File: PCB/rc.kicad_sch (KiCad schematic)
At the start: 5 parts, among them J1 USB_C_Receptacle_USB2.0_16P, J2 USB_A, J3 Conn_01x07_Pin, U1 ESP32-S3-WROOM-1U, U2 MAX3421EEHJ+T

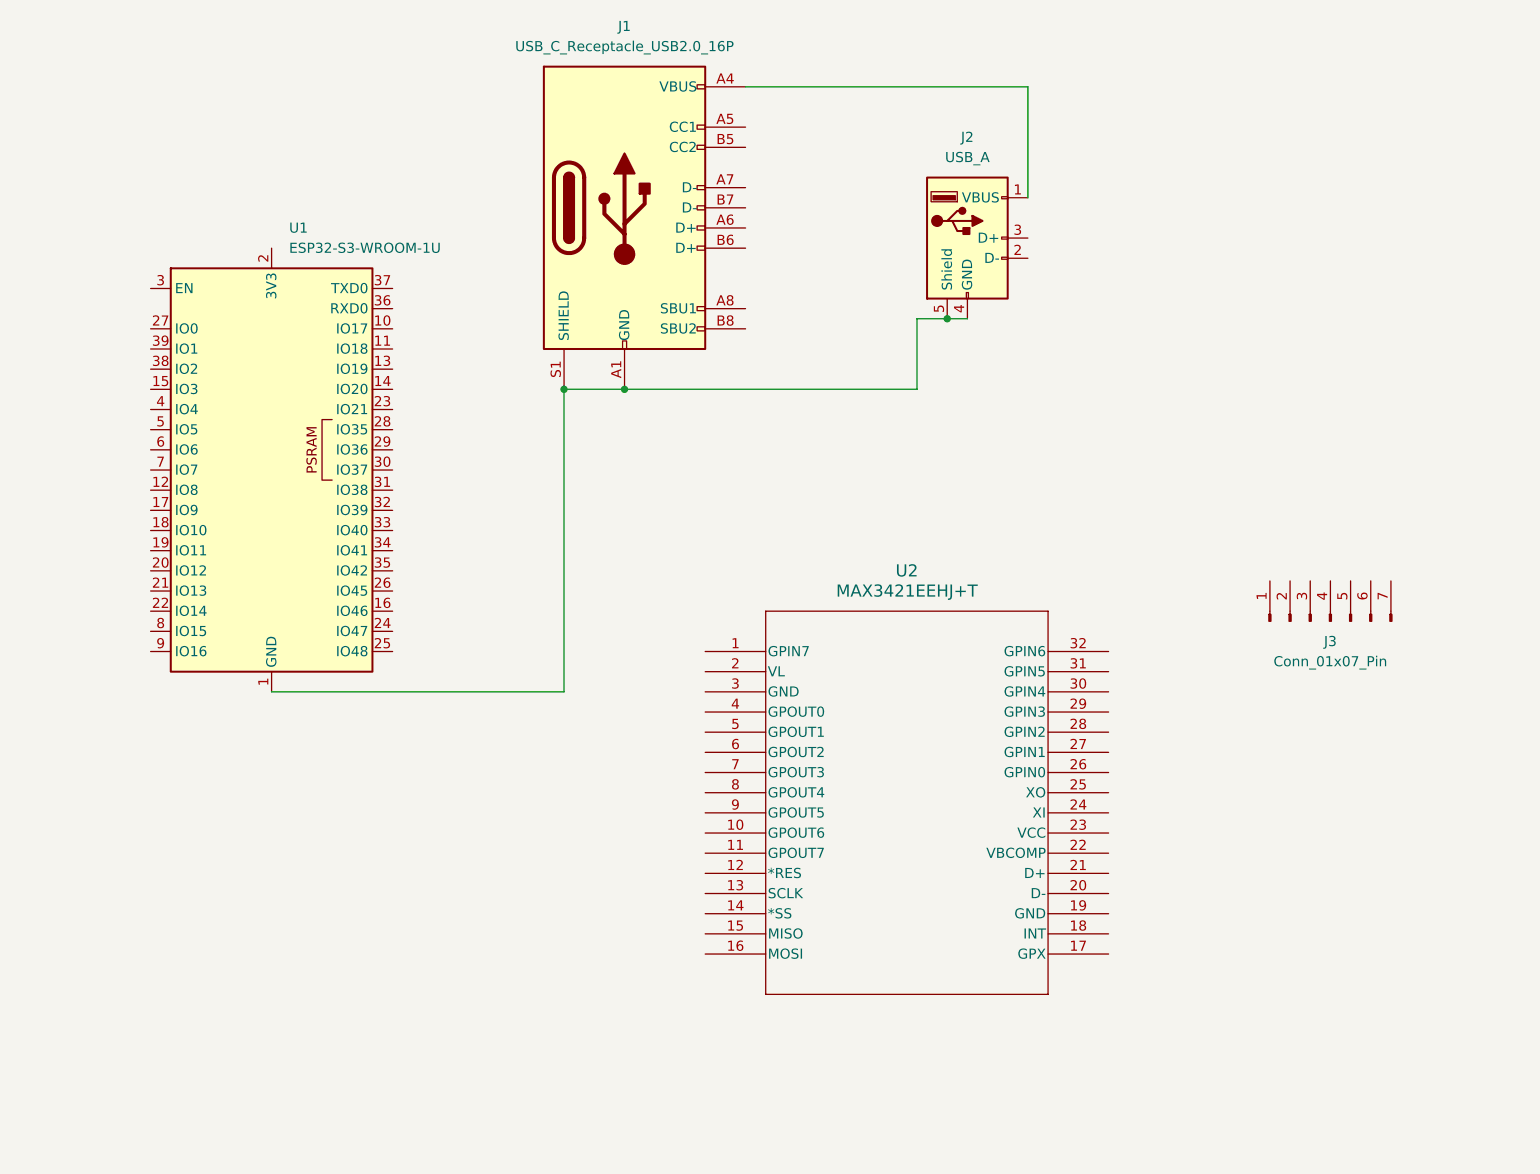
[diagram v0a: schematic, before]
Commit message: pcb init
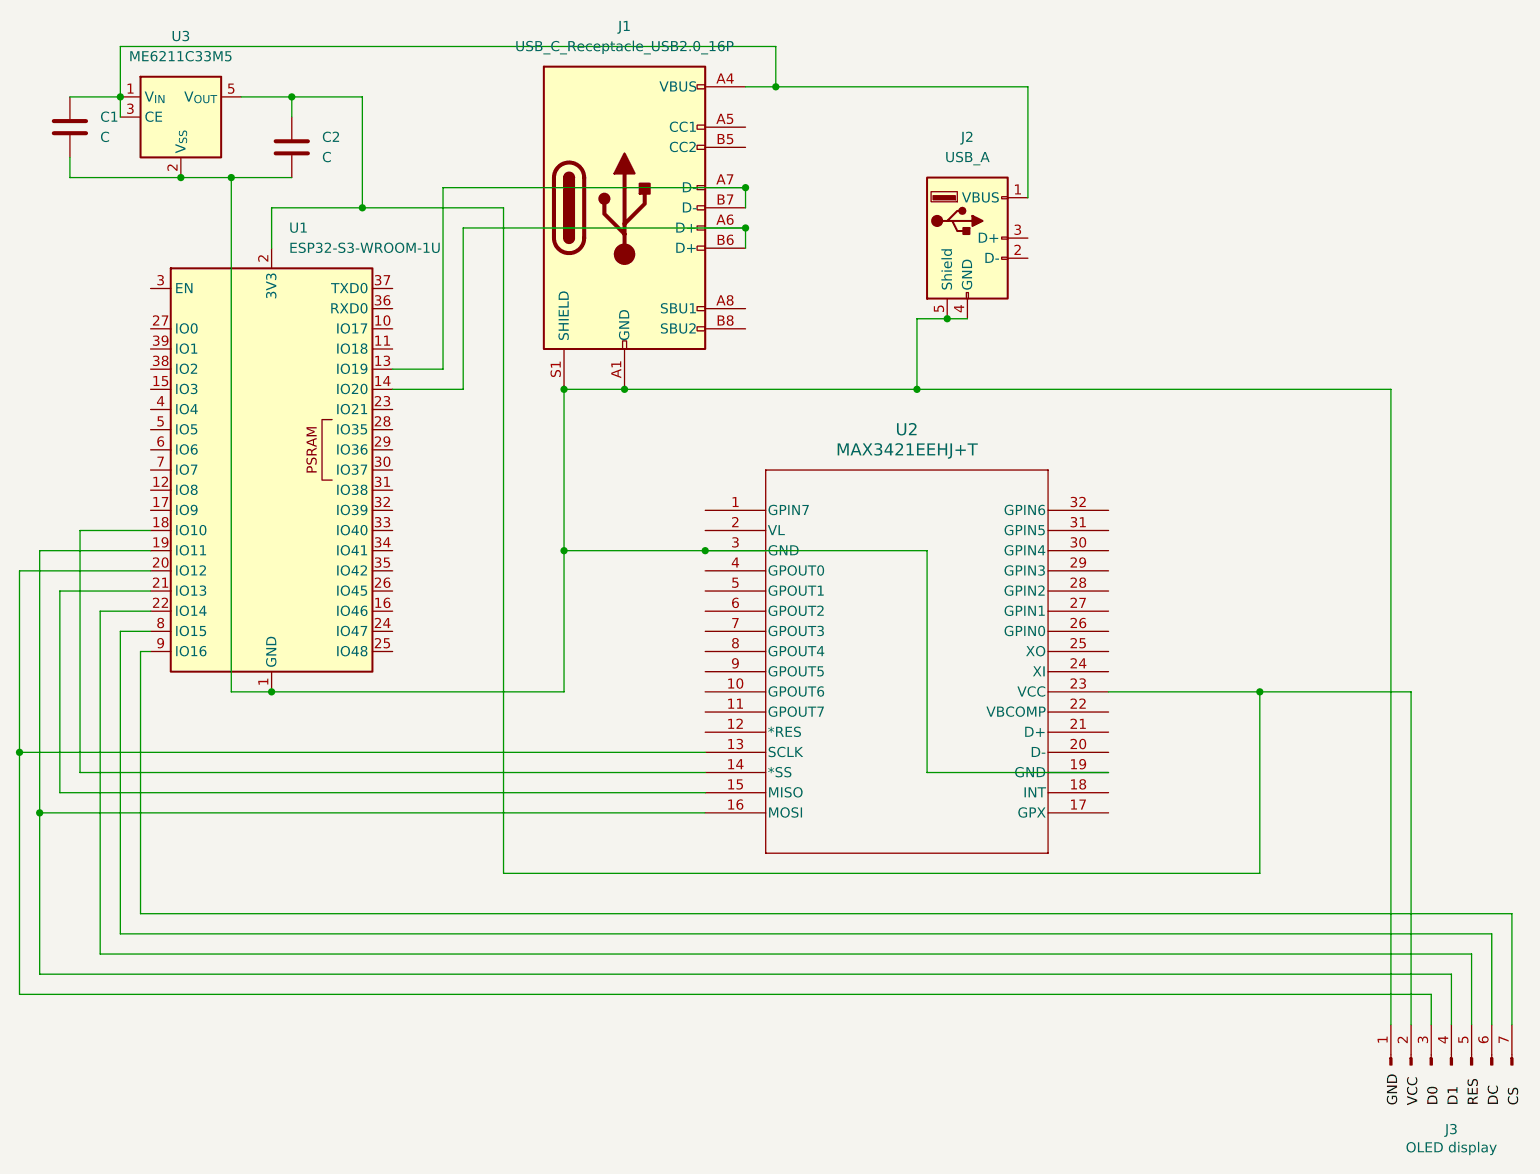
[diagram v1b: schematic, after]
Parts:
- added C1, C2: C, Capacitor_SMD:C_0402_1005Metric_Pad0.74x0.62mm_HandSolder, symbol Device:C
- added U3: ME6211C33M5, Package_TO_SOT_SMD:SOT-23-5, symbol Regulator_Linear:ME6211C33M5
- J3: value Conn_01x07_Pin -> OLED display
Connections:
- net at J1.A1 (GND), J1.A12 (GND), J1.B1 (GND)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: now also J3.1 (Pin_1), U2.19 (GND), U2.3 (GND), C1.2, C2.2, U3.2 (V_{SS})
- net at J1.A4 (VBUS), J1.A9 (VBUS), J1.B4 (VBUS)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: now also C1.1, U3.1 (V_{IN}), U3.3 (CE)
- net at J1.A6 (D+): now also J1.B6 (D+), U1.14 (IO20)
- net at J1.A7 (D-): now also J1.B7 (D-), U1.13 (IO19)
- net at U1.18 (IO10): now also U2.14 (*SS)
- net at U1.19 (IO11): now also J3.4 (Pin_4), U2.16 (MOSI)
- net at U1.2 (3V3): now also J3.2 (Pin_2), U2.23 (VCC), C2.1, U3.5 (V_{OUT})
- net at U1.20 (IO12): now also J3.3 (Pin_3), U2.13 (SCLK)
- net at U1.21 (IO13): now also U2.15 (MISO)
- net at U1.22 (IO14): now also J3.5 (Pin_5)
- net at U1.8 (IO15): now also J3.6 (Pin_6)
- net at U1.9 (IO16): now also J3.7 (Pin_7)
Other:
- moved on the sheet: J3, U2
